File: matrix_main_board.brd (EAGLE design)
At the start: 155.7 x 92.3 mm, 137 parts, among them IC2 24AA01SM, IC3 74HC595D, IC4 74HC595D, IC5 74HC595D, IC6 74HC595D, IC7 NPIC6C596, IC8 NPIC6C596, IC9 W25Q128

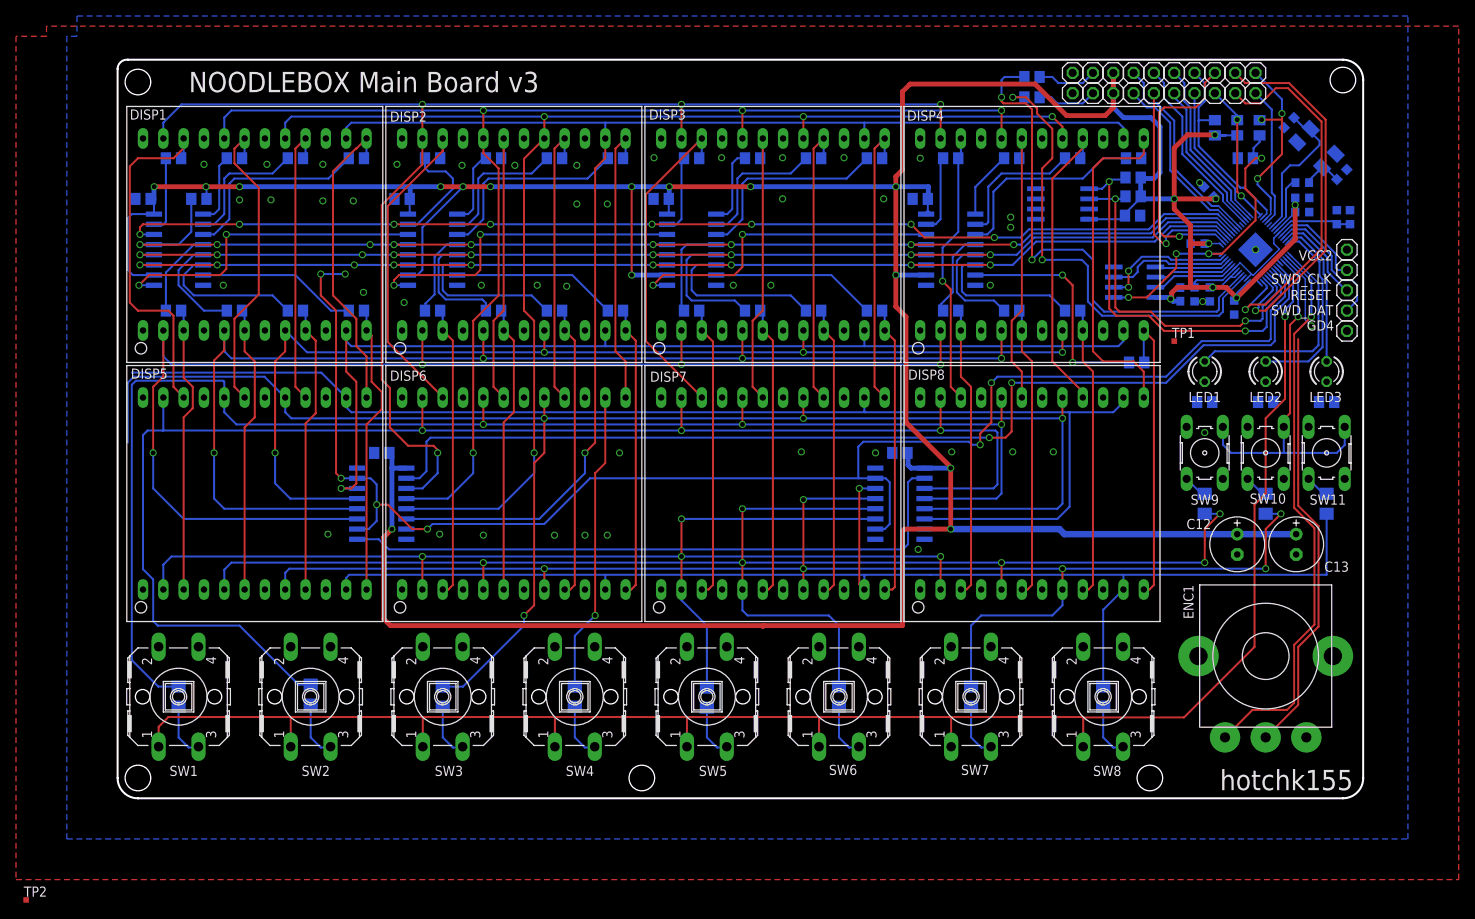
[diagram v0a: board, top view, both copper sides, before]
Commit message: Rolling back RP2040 changes
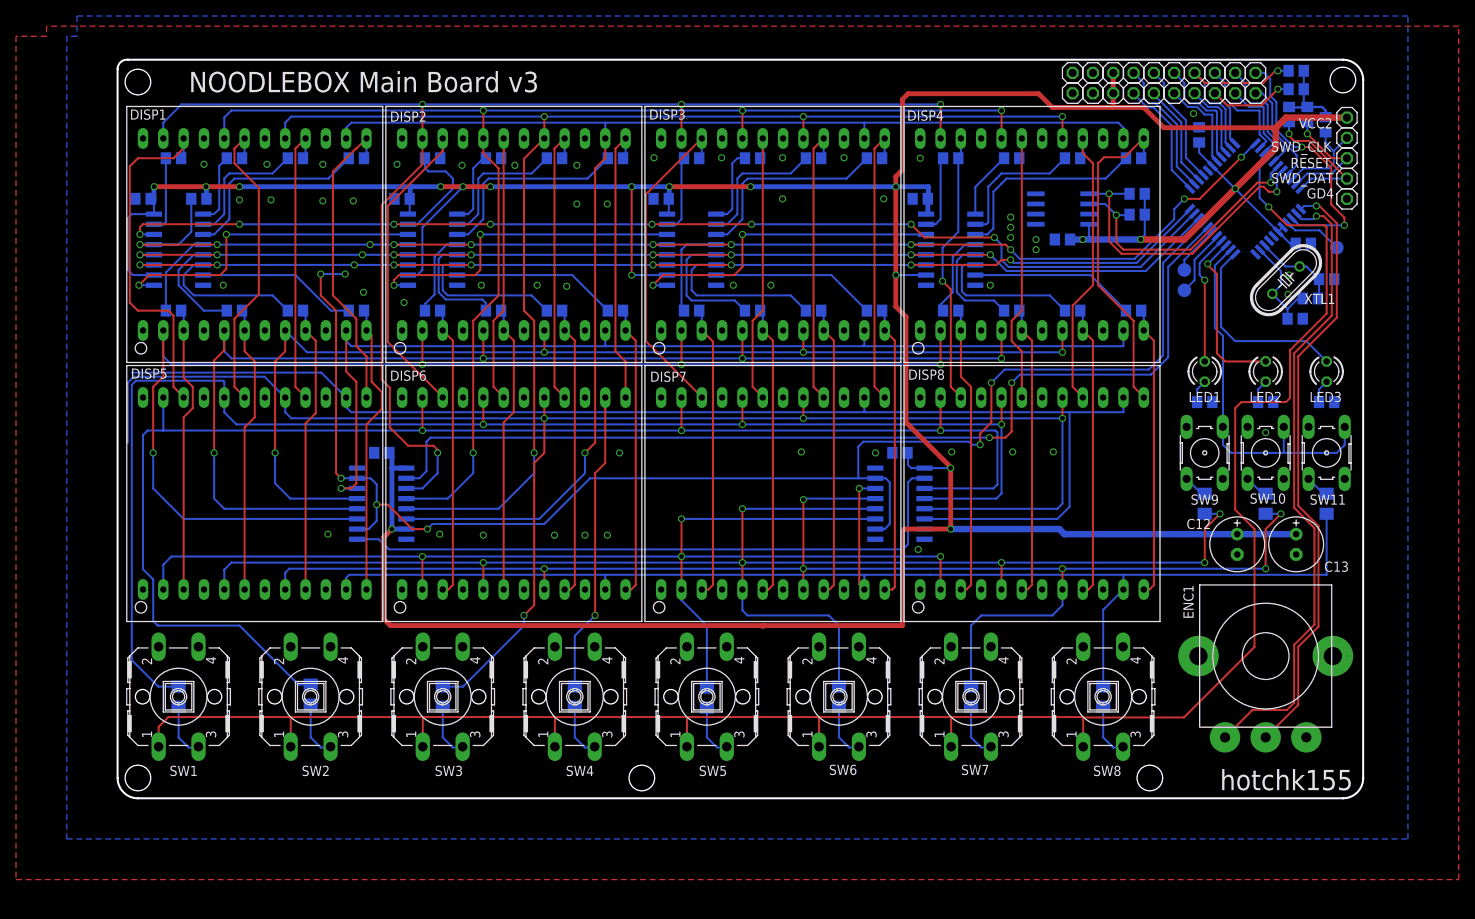
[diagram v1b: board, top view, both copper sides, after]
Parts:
- removed C14, C15: 18p, rcl:C0603K
- removed C16: 100n, resistor:C0603
- removed C17, C18, C20, C22, C23, C26, C27: (no value), rcl:C0603K
- removed C24, C25: 1u, rcl:C0603K
- removed D+: (no value), pinhead:1X01
- removed IC9: W25Q128, jason_eagle6:SO08
- removed Q1: (no value), adafruit:CTS406
- removed R45: (no value), rcl:R0603
- removed R46, R47: (no value), rcl:R0805
- removed TP1, TP2: TPTP07SQ, testpad:TP07SQ
- removed U$1: RP2040, jason_eagle6:QFN40P700X700X90-57N
- added C1, C4: (no value), rcl:C0805
- added C11, C2: 18p, rcl:C0805
- added GD3: (no value), pinhead:1X01
- added IC1: MKE02_44PIN, jason_eagle6:TQFP44
- added PD6, PD7, PH2: TPTP17R, testpad:TP17R
- added R5, R6: (no value), rcl:R0805
- added XTL1: 20m, crystal:HC49/S
- moved R3 34.7 mm to (150.0, 89.3), turned to 90 degrees
- moved R4 32.2 mm to (147.7, 89.3), turned to 90 degrees
- moved SWD_CLK 16.5 mm to (154.9, 86.4)
- moved SWD_DAT 16.5 mm to (154.9, 81.3)
- moved VCC2 16.5 mm to (154.9, 88.9)
- moved GD4 16.5 mm to (154.9, 78.7)
- moved RESET 16.5 mm to (154.9, 83.8)
- moved C3 13.1 mm to (136.5, 86.7), turned to 270 degrees
- moved R43 12.4 mm to (148.6, 94.7), turned to 180 degrees
- moved R44 8.81 mm to (148.6, 92.5), turned to 180 degrees
- moved R26 6.49 mm to (128.3, 64.8)
- moved GD1 3.59 mm to (123.2, 94.5)
- moved R1 2.34 mm to (128.7, 76.8)
- moved R2 2.09 mm to (128.7, 79.4)
- moved IC2 0.64 mm to (119.4, 77.5)
- renumbered D- to GD5
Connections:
- removed net +1V1: C25.2, C26.2, C27.2, U$1.23, U$1.45, U$1.50
- removed net +3V3: C10.2, C12.+, C13.+, C16.2, C17.2, C18.2, C20.2, C22.2, C23.2, C24.2, C3.2, C5.2, C6.2, C7.2, C8.2, C9.2, IC2.8, IC3.10, IC3.16, IC4.10, IC4.16, IC5.10, IC5.16, IC6.10, IC6.16, IC7.1, IC7.7, IC8.1, IC8.7, IC9.8, R1.2, R2.2, R42.2, R43.2, R44.2, R46.1, U$1.1, U$1.10, U$1.22, U$1.33, U$1.42, U$1.43, U$1.44, U$1.48, U$1.49, VCC.1, VCC1.1
- removed net N$10: C14.2, Q1.3, U$1.20
- removed net N$12: C15.2, Q1.1, R45.2
- removed net N$15: R45.1, U$1.21
- removed net N$25: GD5.1, R4.2
- removed net N$26: TP2.TP, U$1.19
- removed net N$65: TP1.TP, U$1.37
- removed net QSPI_CSN: IC9.1, R46.2, R47.2, U$1.56
- removed net QSPI_SCLK: IC9.6, U$1.52
- removed net QSPI_SD0: IC9.5, U$1.53
- removed net QSPI_SD1: IC9.2, U$1.55
- removed net QSPI_SD2: IC9.3, U$1.54
- removed net QSPI_SD3: IC9.7, U$1.51
- removed net SWD_CLK: SWD_CLK.1, U$1.24
- removed net SWD_DAT: SWD_DAT.1, U$1.25
- removed net SWD_RESET: RESET.1, U$1.26
- removed net USB_DM: R4.1, U$1.46
- removed net USB_DP: R3.1, U$1.47
- new net +5V: C1.2, C10.2, C12.+, C13.+, C3.2, C4.2, C5.2, C6.2, C7.2, C8.2, C9.2, IC1.28, IC1.5, IC1.6, IC2.8, IC3.10, IC3.16, IC4.10, IC4.16, IC5.10, IC5.16, IC6.10, IC6.16, IC7.1, IC7.7, IC8.1, IC8.7, R1.2, R2.2, R3.2, R4.2, R42.2, R43.2, R44.2, R5.2, VCC.1, VCC1.1, VCC2.1
- new net NRESET: IC1.43, R3.1, RESET.1
- new net PTD6: IC1.17, PD6.TP
- new net PTD7: IC1.16, PD7.TP
- new net PTH2: IC1.4, PH2.TP
- new net SWDCLK: IC1.42, R5.1, SWD_CLK.1
- new net SWDIO: IC1.44, R4.1, SWD_DAT.1
- net AUXIN: now also IC1.36; no longer U$1.41
- net AUXOUT: now also IC1.25; no longer U$1.3
- net D_ACK: now also IC1.22; no longer U$1.4
- net D_ADT: now also IC1.21; no longer U$1.7
- net D_ARK: now also IC1.20; no longer U$1.5
- net D_ENA: now also IC1.34; no longer U$1.6
- net D_KCK: now also IC1.19; no longer U$1.36
- net D_KDT: now also IC1.18; no longer U$1.35
- net ENC1: now also IC1.1; no longer U$1.31
- net ENC2: now also IC1.2; no longer U$1.30
- net GATE1: now also IC1.31; no longer U$1.14
- net GATE2: now also IC1.30; no longer U$1.13
- net GATE3: now also IC1.29; no longer U$1.12
- net GATE4: now also IC1.26; no longer U$1.11
- net GND: now also C1.1, C11.1, C2.1, C4.1, GD3.1, GD5.1, IC1.11, IC1.27, IC1.8; no longer C14.1, C15.1, C16.1, C17.1, C18.1, C20.1, C22.1, C23.1, C24.1, C25.1, C26.1, C27.1, IC9.4, U$1.57
- net I2C0SCL: now also IC1.32; no longer U$1.16
- net I2C0SDA: now also IC1.33; no longer U$1.15
- net I2C1SCL: now also IC1.39; no longer U$1.39
- net I2C1SDA: now also IC1.40; no longer U$1.38
- net KEY_READ1: now also IC1.37; no longer U$1.34
- net KEY_READ2: now also IC1.13; no longer U$1.32
- net LED1: now also IC1.12; no longer U$1.27
- net LED2: now also IC1.14; no longer U$1.28
- net LED3: now also IC1.15; no longer U$1.29
- net MIDIRX: now also IC1.24; no longer U$1.9
- net MIDITX: now also IC1.23; no longer U$1.8
- net N$4: now also C2.2, IC1.9, R6.2, XTL1.2; no longer VCC2.1
- net N$5: now also C11.2, IC1.10, R6.1, XTL1.1; no longer D+.1, R3.2
- net OFF_SW: now also IC1.3; no longer R47.1, U$1.17
- net PWR_CTRL: now also IC1.38; no longer U$1.40
- net SYNCIN: now also IC1.35; no longer U$1.2
- net SYNCOUT: now also IC1.41; no longer U$1.18
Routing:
- net +3V3: track 541.1 -> 0.00 mm, vias 23 -> 0
- net +5V: track 0.00 -> 517.8 mm, vias 0 -> 18
- net USB_DP: track 64.4 -> 0.00 mm, vias 2 -> 0
- net USB_DM: track 59.1 -> 0.00 mm, vias 2 -> 0
- net QSPI_CSN: track 38.5 -> 0.00 mm, vias 4 -> 0
- net AUXIN: track 47.2 -> 10.8 mm, vias 1 -> 0
- net PWR_CTRL: track 47.2 -> 15.4 mm, vias 1 -> 0
- net +1V1: track 27.6 -> 0.00 mm
- net KEY_READ1: track 220.1 -> 246.7 mm
- net SYNCIN: track 33.9 -> 14.0 mm, vias 1 -> 0
- net N$10: track 19.2 -> 0.00 mm
- net SWDIO: track 0.00 -> 17.5 mm, vias 0 -> 1
- net SWD_DAT: track 17.4 -> 0.00 mm
- net QSPI_SD1: track 16.9 -> 0.00 mm, vias 2 -> 0
- net AUXOUT: track 28.9 -> 13.2 mm, vias 1 -> 0
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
